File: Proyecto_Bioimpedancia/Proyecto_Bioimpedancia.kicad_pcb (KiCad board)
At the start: 2 copper layers, 61 x 33.3 mm, 59 parts, among them J1 Jumper_Calibration, J2 Jumper, J3 Jumper, J4 Jumper, P1 CONN_01X03, P2 CONN_01X02, P3 CONN_01X02, P4 CONN_01X02, P5 CONN_01X02, P6 CONN_01X02, P7 CONN_01X02, SW1 SW_PUSH, U1 AD8606, U2 ADG819, U3 Atmega328PA, U4 KC5032A_CM, U5 ADP3334, Y1 AMB3_16M

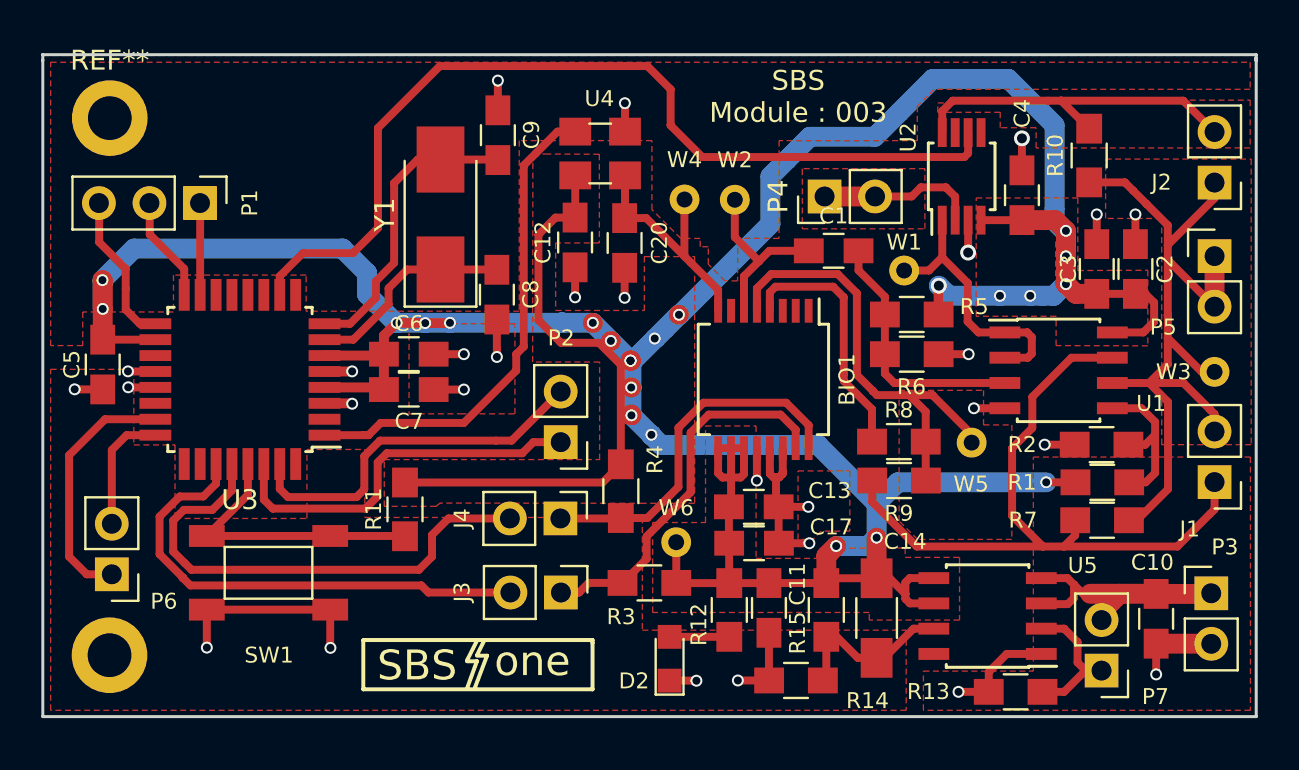
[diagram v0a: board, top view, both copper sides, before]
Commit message: Diseño Final con Planos Expandidos
Diseño 18 de Mayo
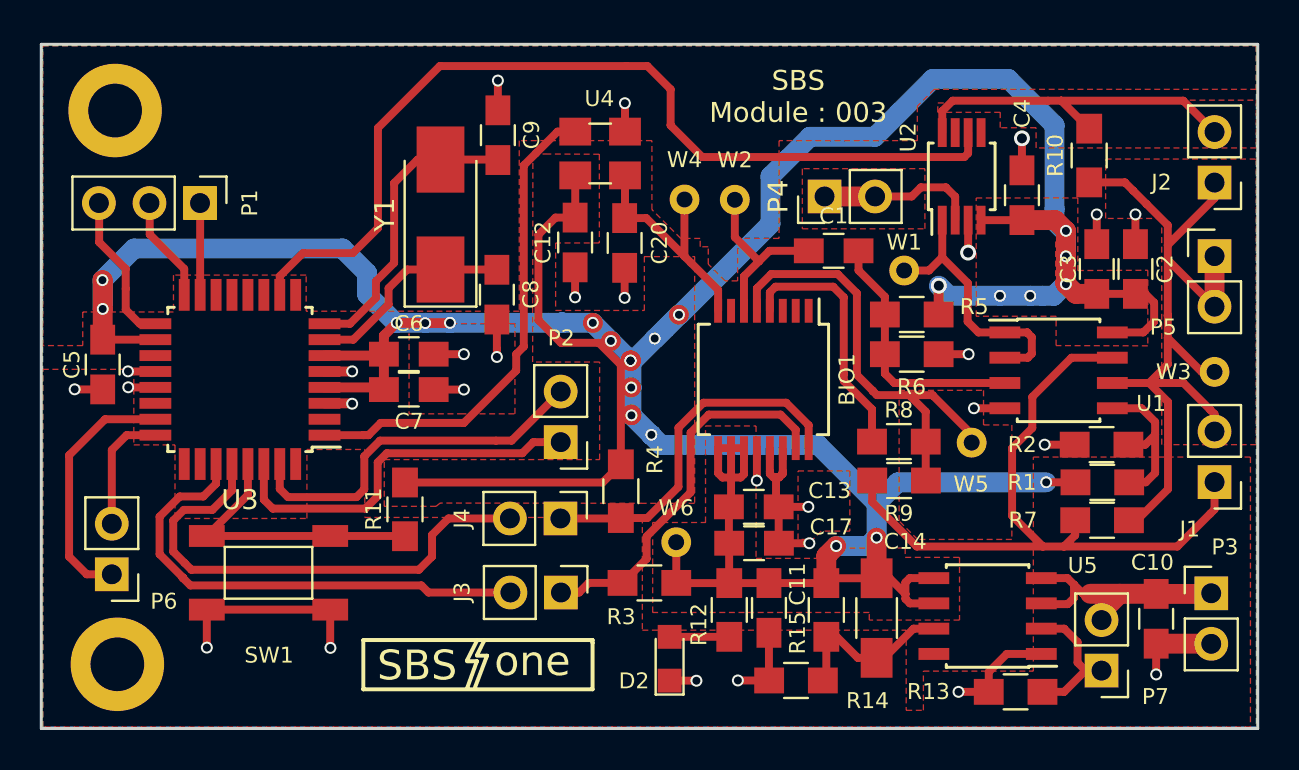
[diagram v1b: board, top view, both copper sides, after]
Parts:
- removed the REF** at (179.5, 82.1)
- added REF**: MountingHole_2.2mm_M2_DIN965_Pad, Mounting_Holes:MountingHole_2.7mm_M2.5_DIN965_Pad, F.Cu at (179.9, 82.6)
- REF**: footprint Mounting_Holes:MountingHole_2.2mm_M2_DIN965_Pad -> Mounting_Holes:MountingHole_2.7mm_M2.5_DIN965_Pad
- moved REF** 0.47 mm to (179.8, 54.8)
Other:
- board size 61 x 33.3 mm -> 61.1 x 34.4 mm
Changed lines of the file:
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@@
     (links 124)
     (no_connects 0)
-    (area 176.099399 51.880699 237.234801 85.292001)
+    (area 165.072814 51.359999 242.483768 88.10912)
     (thickness 1.6)
-    (drawings 23)
+    (drawings 18)
     (tracks 590)
     (zones 0)
@@
   )
   (setup
-    (last_trace_width 0.4)
+    (last_trace_width 0.1778)
     (user_trace_width 0.4)
     (user_trace_width 0.5)
@@
     (visible_elements 7FFEFFFF)
     (pcbplotparams
-      (layerselection 0x01030_80000001)
+      (layerselection 0x3ffff_80000001)
       (usegerberextensions false)
       (excludeedgelayer true)
@@
       (drillshape 0)
       (scaleselection 1)
-      (outputdirectory Gerber/))
+      (outputdirectory ../../Gerber/Andres/))
   )
   (net 0 "")
@@
     (add_net "Net-(U5-Pad8)")
   )
-  (module Mounting_Holes:MountingHole_2.2mm_M2_DIN965_Pad (layer F.Cu)
-    (at 179.5526 55.1434)
-    (descr "Mounting Hole 2.2mm, M2, DIN965")
-    (tags "mounting hole 2.2mm m2 din965")
-    (fp_text reference REF** (at 0 -2.9) (layer F.SilkS)
-      (effects (font (size 1 1) (thickness 0.15)))
-    )
-    (fp_text value MountingHole_2.2mm_M2_DIN965_Pad (at 0 2.9) (layer F.Fab)
-      (effects (font (size 1 1) (thickness 0.15)))
-    )
-    (fp_circle (center 0 0) (end 1.9 0) (layer Cmts.User) (width 0.15))
-    (fp_circle (center 0 0) (end 2.15 0) (layer F.CrtYd) (width 0.05))
-    (pad 1 thru_hole circle (at 0 0) (size 3.8 3.8) (drill 2.2) (layers *.Cu *.Mask))
+  (module Mounting_Holes:MountingHole_2.7mm_M2.5_DIN965_Pad (layer F.Cu)
+    (at 179.9336 82.5881)
+    (descr "Mounting Hole 2.7mm, M2.5, DIN965")
+    (tags "mounting hole 2.7mm m2.5 din965")
+    (fp_text reference REF** (at 5.1689 1.5494) (layer F.SilkS) hide
+      (effects (font (size 1 1) (thickness 0.15)))
+    )
+    (fp_text value MountingHole_2.2mm_M2_DIN965_Pad (at 0 3.35) (layer F.Fab)
+      (effects (font (size 1 1) (thickness 0.15)))
+    )
+    (fp_circle (center 0 0) (end 2.35 0) (layer Cmts.User) (width 0.15))
+    (fp_circle (center 0 0) (end 2.6 0) (layer F.CrtYd) (width 0.05))
+    (pad 1 thru_hole circle (at 0 0) (size 4.7 4.7) (drill 2.7) (layers *.Cu *.Mask))
   )
   (module Housings_SSOP:SSOP-16_5.3x6.2mm_Pitch0.65mm (layer F.Cu)
@@
     )
   )
-  (module Mounting_Holes:MountingHole_2.2mm_M2_DIN965_Pad (layer F.Cu)
-    (at 179.5399 82.1309)
-    (descr "Mounting Hole 2.2mm, M2, DIN965")
-    (tags "mounting hole 2.2mm m2 din965")
-    (fp_text reference REF** (at 4.953 1.651) (layer F.SilkS) hide
-      (effects (font (size 1 1) (thickness 0.15)))
-    )
-    (fp_text value MountingHole_2.2mm_M2_DIN965_Pad (at 0 2.9) (layer F.Fab)
-      (effects (font (size 1 1) (thickness 0.15)))
-    )
-    (fp_circle (center 0 0) (end 1.9 0) (layer Cmts.User) (width 0.15))
-    (fp_circle (center 0 0) (end 2.15 0) (layer F.CrtYd) (width 0.05))
-    (pad 1 thru_hole circle (at 0 0) (size 3.8 3.8) (drill 2.2) (layers *.Cu *.Mask))
-  )
+  (module Mounting_Holes:MountingHole_2.7mm_M2.5_DIN965_Pad (layer F.Cu)
+    (at 179.8193 54.7624)
+    (descr "Mounting Hole 2.7mm, M2.5, DIN965")
+    (tags "mounting hole 2.7mm m2.5 din965")
+    (fp_text reference REF** (at 5.3086 0.0254) (layer F.SilkS) hide
+      (effects (font (size 1 1) (thickness 0.15)))
+    )
+    (fp_text value MountingHole_2.2mm_M2_DIN965_Pad (at 0 3.35) (layer F.Fab)
+      (effects (font (size 1 1) (thickness 0.15)))
+    )
+    (fp_circle (center 0 0) (end 2.35 0) (layer Cmts.User) (width 0.15))
+    (fp_circle (center 0 0) (end 2.6 0) (layer F.CrtYd) (width 0.05))
+    (pad 1 thru_hole circle (at 0 0) (size 4.7 4.7) (drill 2.7) (layers *.Cu *.Mask))
+  )
+  (gr_line (start 176.1109 85.8139) (end 176.1109 51.435) (angle 90) (layer Edge.Cuts) (width 0.15))
+  (gr_line (start 176.1109 51.435) (end 237.236 51.435) (angle 90) (layer Edge.Cuts) (width 0.15))
+  (gr_line (start 237.236 85.8139) (end 176.1109 85.8139) (angle 90) (layer Edge.Cuts) (width 0.15))
+  (gr_line (start 237.236 51.435) (end 237.236 85.8139) (angle 90) (layer Edge.Cuts) (width 0.15))
   (gr_text "SBS\nModule : 003" (at 214.1474 54.0639) (layer F.SilkS)
     (effects (font (size 1 1) (thickness 0.2)))
@@
     (effects (font (size 1.5 1.5) (thickness 0.375)))
   )
-  (gr_line (start 237.1598 52.2605) (end 237.1471 52.2605) (angle 90) (layer Edge.Cuts) (width 0.15))
-  (gr_line (start 237.1598 51.9557) (end 237.1598 52.2605) (angle 90) (layer Edge.Cuts) (width 0.15))
-  (gr_line (start 176.1744 51.9557) (end 237.1598 51.9557) (angle 90) (layer Edge.Cuts) (width 0.15))
-  (gr_line (start 176.1871 51.9684) (end 176.1744 51.9557) (angle 90) (layer Edge.Cuts) (width 0.15))
-  (gr_line (start 176.1871 52.2605) (end 176.1871 51.9684) (angle 90) (layer Edge.Cuts) (width 0.15))
-  (gr_line (start 237.1344 52.2224) (end 237.1344 52.1208) (angle 90) (layer Edge.Cuts) (width 0.15))
-  (gr_line (start 176.1871 85.217) (end 176.1871 52.2224) (angle 90) (layer Edge.Cuts) (width 0.15))
-  (gr_line (start 237.1598 85.217) (end 176.1871 85.217) (angle 90) (layer Edge.Cuts) (width 0.15))
-  (gr_line (start 237.1598 52.1335) (end 237.1598 85.217) (angle 90) (layer Edge.Cuts) (width 0.15))
   (segment (start 216.4334 68.0085) (end 216.4334 68.3514) (width 0.4) (layer F.Cu) (net 1))
   (segment (start 212.7198 64.8252) (end 212.7198 63.8989) (width 0.4) (layer F.Cu) (net 1))
@@
   (segment (start 232.1306 79.0521) (end 234.8665 79.0521) (width 1) (layer F.Cu) (net 12))
   (segment (start 234.8665 79.0521) (end 234.8992 79.0194) (width 1) (layer F.Cu) (net 12))
-  (segment (start 235.0643 73.4314) (end 235.0643 74.803) (width 0.4) (layer F.Cu) (net 13) (status 400000))
+  (segment (start 235.0643 73.4314) (end 235.0643 74.803) (width 0.4) (layer F.Cu) (net 13))
   (segment (start 233.1974 76.6699) (end 234.8484 75.0189) (width 0.4) (layer F.Cu) (net 13))
   (segment (start 233.1974 76.6699) (end 227.4951 76.6699) (width 0.4) (layer F.Cu) (net 13))
@@
   (segment (start 226.441 76.6699) (end 227.4951 76.6699) (width 0.4) (layer F.Cu) (net 13))
   (segment (start 224.8916 75.1205) (end 226.441 76.6699) (width 0.4) (layer F.Cu) (net 13))
-  (segment (start 235.0643 70.8914) (end 235.0643 70.0151) (width 0.4) (layer F.Cu) (net 14) (status 400000))
+  (segment (start 235.0643 70.8914) (end 235.0643 70.0151) (width 0.4) (layer F.Cu) (net 14))
   (segment (start 233.5022 68.453) (end 234.8484 69.7992) (width 0.4) (layer F.Cu) (net 14))
   (segment (start 233.2101 68.453) (end 231.775 68.453) (width 0.4) (layer F.Cu) (net 14))
@@
     (polygon
       (pts
-        (xy 176.1998 51.9938) (xy 237.1598 51.9938) (xy 237.1598 85.1916) (xy 176.1871 85.1916) (xy 176.1871 51.9938)
+        (xy 237.1598 85.7377) (xy 176.1871 85.7377) (xy 176.1871 51.5112) (xy 237.1598 51.5112) (xy 237.1598 85.7377)
       )
     )
@@
     (polygon
       (pts
-        (xy 236.855 53.6956) (xy 220.98 53.6956) (xy 220.1291 54.5465) (xy 220.1291 56.2737) (xy 213.1822 56.2737)
+        (xy 237.1598 53.6956) (xy 220.98 53.6956) (xy 220.1291 54.5465) (xy 220.1291 56.2737) (xy 213.1822 56.2737)
         (xy 213.1822 61.1886) (xy 211.0994 61.1886) (xy 211.0994 63.3222) (xy 210.4644 63.3222) (xy 209.6262 62.484)
         (xy 209.6262 61.6077) (xy 209.2198 61.6077) (xy 209.2198 61.1886) (xy 208.2419 61.1886) (xy 206.7941 59.7408)
         (xy 206.7941 56.2737) (xy 200.1266 56.2737) (xy 200.1266 64.8462) (xy 189.4205 64.8462) (xy 189.4205 63.0301)
-        (xy 182.753 63.0301) (xy 182.753 64.8843) (xy 178.1937 64.8843) (xy 178.1937 66.5734) (xy 176.5808 66.5734)
-        (xy 176.5808 52.3367) (xy 236.855 52.3367) (xy 236.855 53.6956)
+        (xy 182.753 63.0301) (xy 182.753 64.8843) (xy 178.1937 64.8843) (xy 178.1937 66.5734) (xy 176.1871 66.5734)
+        (xy 176.1871 51.5112) (xy 237.1598 51.5112) (xy 237.1598 53.6956)
       )
     )
@@
     (polygon
       (pts
-        (xy 236.9058 71.5518) (xy 232.41 71.5518) (xy 232.41 60.1853) (xy 229.5906 60.1853) (xy 229.5906 57.2008)
-        (xy 236.9058 57.2008) (xy 236.9058 71.5518)
+        (xy 237.1598 71.5518) (xy 232.41 71.5518) (xy 232.41 60.1853) (xy 229.5906 60.1853) (xy 229.5906 57.2008)
+        (xy 237.1598 57.2008) (xy 237.1598 71.5518)
       )
     )
@@
     (polygon
       (pts
-        (xy 236.855 56.642) (xy 226.0981 56.642) (xy 226.0981 55.626) (xy 224.2947 55.626) (xy 224.2947 54.8513)
-        (xy 221.1578 54.8513) (xy 221.1578 54.3814) (xy 226.0981 54.3814) (xy 226.0981 54.2417) (xy 236.855 54.2417)
-        (xy 236.855 56.642)
+        (xy 237.1598 56.642) (xy 226.0981 56.642) (xy 226.0981 55.626) (xy 224.2947 55.626) (xy 224.2947 54.8513)
+        (xy 221.1578 54.8513) (xy 221.1578 54.3814) (xy 226.0981 54.3814) (xy 226.0981 54.2417) (xy 237.1598 54.2417)
+        (xy 237.1598 56.642)
       )
     )
@@
         (xy 180.7591 71.5645) (xy 182.8292 71.5645) (xy 182.8292 75.2602) (xy 189.4586 75.2602) (xy 189.4586 71.7931)
         (xy 192.3669 71.7931) (xy 192.3669 75.2094) (xy 206.3115 75.2094) (xy 206.3115 80.8736) (xy 219.5703 80.8736)
-        (xy 219.5703 84.8995) (xy 176.5808 84.8995) (xy 176.5808 67.7672) (xy 180.7591 67.7672) (xy 180.7591 71.5645)
+        (xy 219.5703 84.8995) (xy 220.4339 84.8995) (xy 220.4339 82.931) (xy 225.9584 82.931) (xy 225.9584 72.1741)
+        (xy 236.8677 72.1741) (xy 236.8677 85.7377) (xy 176.1871 85.7377) (xy 176.1871 67.7672) (xy 180.7591 67.7672)
+        (xy 180.7591 71.5645)
       )
     )
-  )
-  (zone (net 0) (net_name "") (layer F.Cu) (hatch edge 0.508)
-    (connect_pads yes (clearance 0.508))
-    (min_thickness 0.254)
-    (fill yes (arc_segments 16) (thermal_gap 0.508) (thermal_bridge_width 0.508))
-    (polygon
-      (pts
-        (xy 236.8677 84.8995) (xy 220.4339 84.8995) (xy 220.4339 82.931) (xy 225.9584 82.931) (xy 225.9584 72.1741)
-        (xy 236.8677 72.1741) (xy 236.8677 84.8995)
-      )
-    )
